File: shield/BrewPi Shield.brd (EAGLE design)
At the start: 53.6 x 59.7 mm, 30 parts, among them J1 ARDUINO_R3_SHIELD_ICSP, Q1 2N3906, U1 SN74HC595N

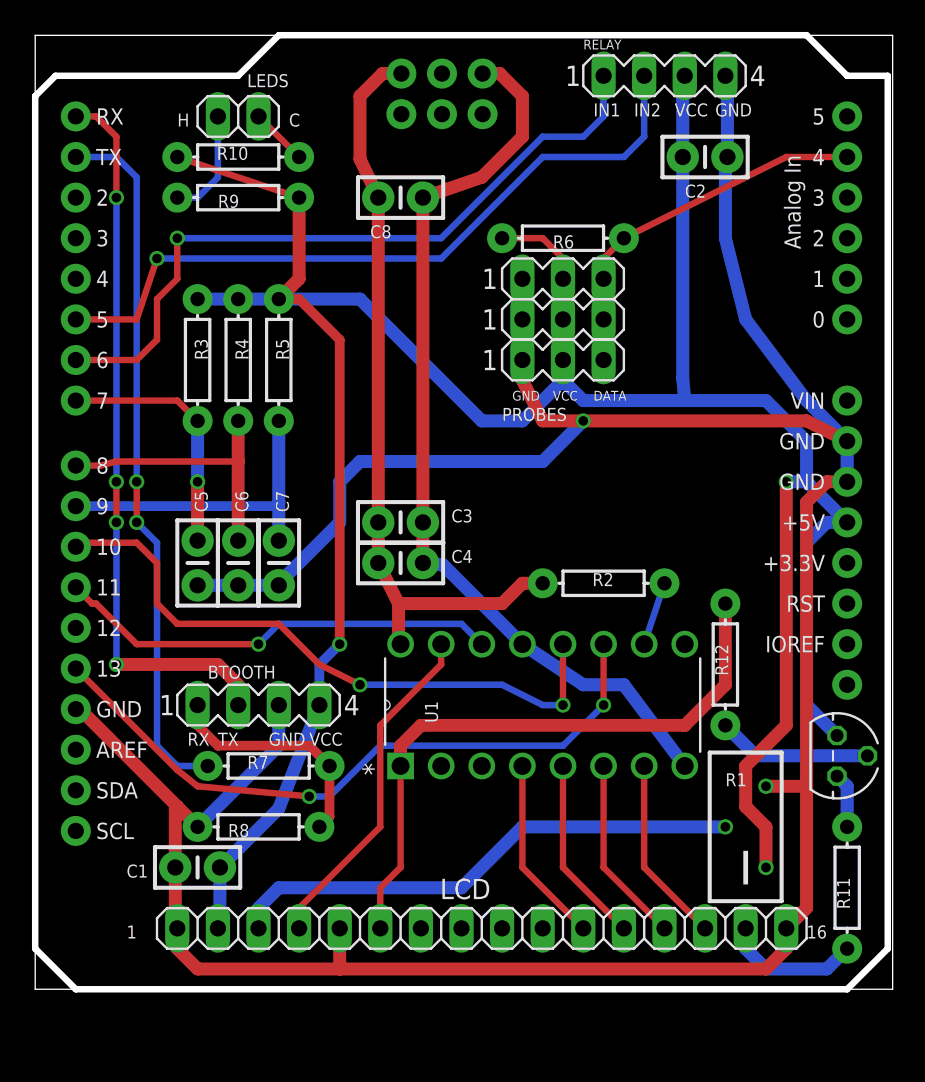
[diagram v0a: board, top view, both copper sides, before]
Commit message: Version 1.3 upload
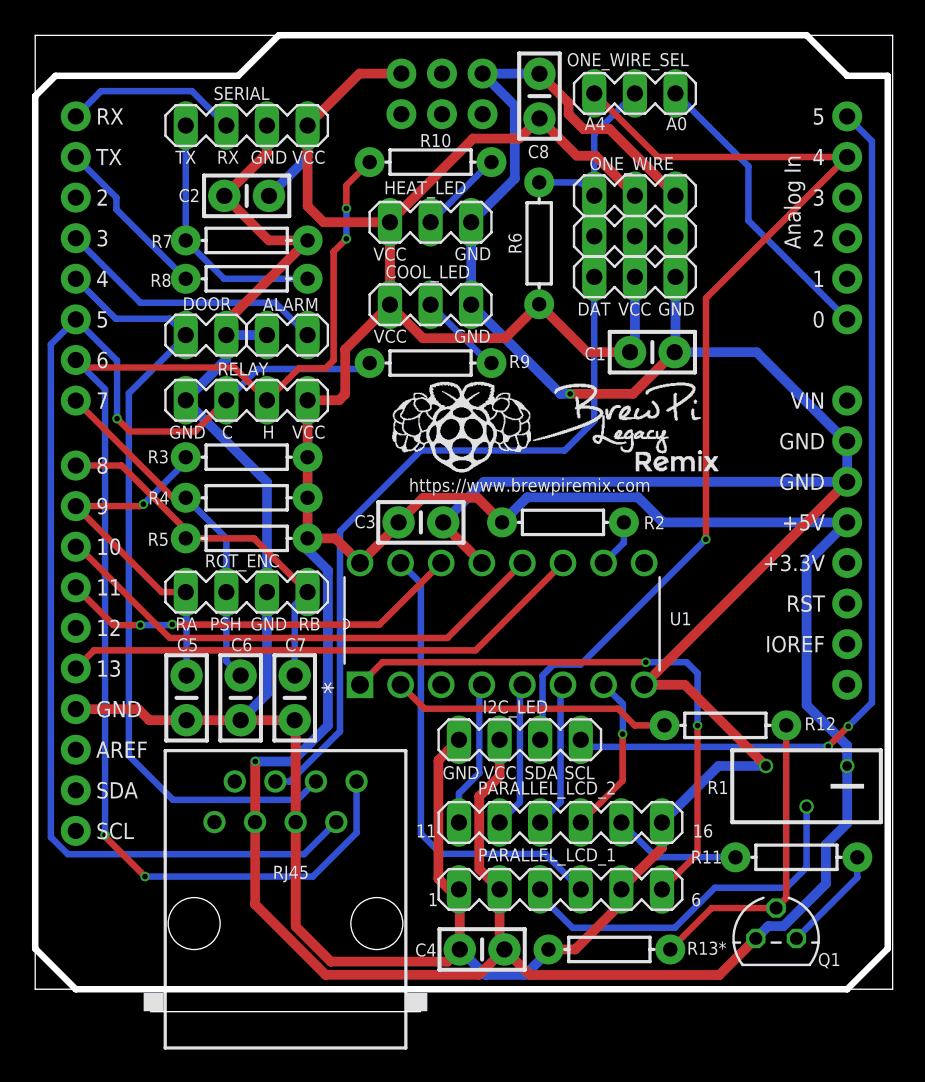
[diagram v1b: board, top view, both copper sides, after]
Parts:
- removed BTOOTH: (no value), con-lstb:MA04-1
- removed LCD: 16 pin, pinhead:1X16
- removed LEDS: (no value), pinhead:1X02
- added ALARM, DOOR: 2 pin, LBussy:HEADER02-1
- added COOL_LED, HEAT_LED, ONE_WIRE_SEL: 3 pin, LBussy:HEADER03-1
- added I2C_LED, ROT_ENC, SERIAL: 4 pin, LBussy:HEADER04-1
- added PARALLEL_LCD_1, PARALLEL_LCD_2: 6 pin, LBussy:HEADER06-1
- added R13*: 10kΩ, SparkFun-Passives:AXIAL-0.3
- added RJ45: RJ45-8X, con-tycoelectronics:RJ45-NO-SHIELD
- C1, C2, C3, C4: value .1UF -> 0.1μF
- C5, C6, C7: value (none) -> 0.1μF
- C8: value 1.0UF -> 1.0μF
- PROBE1, PROBE2, PROBE3: value (none) -> 3 pin; device con-lstb:MA03-1 -> LBussy:HEADER03-1
- R1, R3, R4, R5: value 10K -> 10kΩ
- R10, R9: value 220 -> 220Ω
- R11: value 470 Ohm -> 150Ω
- R12: value 10k Ohm -> 10kΩ
- R2: value 0-20K -> 20kΩ
- R6: value 4.7K -> 4.7kΩ
- R7: value 1K -> 2kΩ
- R8: value 2K -> 1kΩ
- RELAY: value (none) -> 4 pin; device con-lstb:MA04-1 -> LBussy:HEADER04-1
- moved C1 43.0 mm to (62.7, 58.9), turned to 0 degrees
- moved R8 34.3 mm to (37.4, 63.5), turned to 180 degrees
- moved RELAY 33.1 mm to (37.4, 55.9)
- moved R7 32.9 mm to (37.4, 65.9)
- moved C2 28.8 mm to (37.4, 68.7), turned to 180 degrees
- moved C4 24.7 mm to (52.1, 21.5), turned to 180 degrees
- moved R9 15.9 mm to (48.9, 58.2)
- moved Q1 12.0 mm to (70.5, 22.2), turned to 0 degrees
- moved R10 12.0 mm to (48.9, 70.8)
- moved R5 11.3 mm to (37.4, 47.3), turned to 0 degrees
- moved C8 10.8 mm to (55.7, 74.9), turned to 90 degrees
- moved R4 8.64 mm to (37.4, 49.8), turned to 0 degrees
- moved C7 8.50 mm to (40.4, 37.3)
- moved C5 8.47 mm to (33.6, 37.3)
- moved C6 8.44 mm to (37.0, 37.3)
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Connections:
- removed net 5V: BTOOTH.4, C1.1, C2.1, J1.5V, LCD.2, PROBE1.2, PROBE2.2, PROBE3.2, Q1.3, R1.1, R10.P$2, R3.P$2, R4.P$2, R5.P$2, R6.P$1, R9.P$2, RELAY.3
- removed net A5V: C3.1, C4.1, C8.1, J1.5V_ICSP, R2.P$2, U1.16
- removed net AGND: C3.2, C4.2, C8.2, J1.GND_ICSP, U1.13, U1.8
- removed net D5: J1.D5, RELAY.2
- removed net D6: J1.D6, RELAY.1
- removed net D7: C5.1, J1.D7, R3.P$1
- removed net IO8: C6.1, J1.D8, R4.P$1
- removed net IO9: C7.1, J1.D9, R5.P$1
- removed net N$12: LEDS.1, R9.P$1
- removed net N$13: LEDS.2, R10.P$1
- new net 1WIRE: ONE_WIRE_SEL.2, PROBE1.3, PROBE2.3, PROBE3.3, R6.P$2, RJ45.4
- new net A0: J1.A0, ONE_WIRE_SEL.3
- new net A4: I2C_LED.3, J1.A4, ONE_WIRE_SEL.1
- new net A5: I2C_LED.4, J1.A5
- new net ALARM: ALARM.1, J1.D3
- new net COOL: J1.D5, R9.P$1, RELAY.2, RJ45.7
- new net DOOR: DOOR.1, J1.D4, RJ45.6
- new net HEAT: J1.D6, R10.P$2, RELAY.3, RJ45.8
- new net N$8: HEAT_LED.2, R10.P$1
- new net PSHB: C6.1, J1.D7, R4.P$1, ROT_ENC.2
- new net QC: R12.P$1, U1.2
- new net ROTA: C5.1, J1.D9, R3.P$1, ROT_ENC.1
- new net ROTB: C7.1, J1.D8, R5.P$1, ROT_ENC.4
- new net VCC: C1.1, C2.1, C3.1, C4.1, C8.1, COOL_LED.1, HEAT_LED.1, I2C_LED.2, J1.5V, J1.5V_ICSP, PARALLEL_LCD_1.2, PROBE1.2, PROBE2.2, PROBE3.2, Q1.3, R1.1, R2.P$2, R3.P$2, R4.P$2, R5.P$2, R6.P$1, RELAY.4, RJ45.3, SERIAL.4, U1.16
- net GND: now also ALARM.2, C3.2, C4.2, C8.2, COOL_LED.3, DOOR.2, HEAT_LED.3, I2C_LED.1, J1.GND_ICSP, PARALLEL_LCD_1.1, PARALLEL_LCD_1.5, PARALLEL_LCD_2.6, R13*.P$1, R7.P$1, RELAY.1, RJ45.5, ROT_ENC.3, SERIAL.3, U1.13, U1.8; no longer BTOOTH.3, LCD.1, LCD.16, LCD.5, R8.P$1, RELAY.4
- net N$2: now also R13*.P$2
- net N$3: now also R7.P$2, R8.P$1, SERIAL.1; no longer BTOOTH.1, R7.P$1, R8.P$2
- net N$4: now also COOL_LED.2, R9.P$2; no longer J1.A4, PROBE1.3, PROBE2.3, PROBE3.3, R6.P$2
- net N$5: now also PARALLEL_LCD_2.5; no longer LCD.15
- net N$6: now also PARALLEL_LCD_1.3; no longer LCD.3
- net QA: now also PARALLEL_LCD_1.4; no longer LCD.4
- net QB: now also PARALLEL_LCD_1.6; no longer LCD.6, R12.P$1
- net QE: now also PARALLEL_LCD_2.1; no longer LCD.11
- net QF: now also PARALLEL_LCD_2.2; no longer LCD.12
- net QG: now also PARALLEL_LCD_2.3; no longer LCD.13
- net QH: now also PARALLEL_LCD_2.4; no longer LCD.14
- net RX: now also SERIAL.2; no longer BTOOTH.2
- net TX: now also R8.P$2; no longer R7.P$2
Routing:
- net VCC: track 0.00 -> 239.9 mm, vias 0 -> 1
- net 5V: track 184.4 -> 0.00 mm, vias 2 -> 0
- net HEAT: track 0.00 -> 83.2 mm, vias 0 -> 4
- net COOL: track 0.00 -> 77.4 mm, vias 0 -> 1
- net GND: track 198.1 -> 261.7 mm
- net A4: track 0.00 -> 62.9 mm, vias 0 -> 1
- net 1WIRE: track 0.00 -> 62.0 mm
- net AGND: track 57.7 -> 0.00 mm
- net A5: track 0.00 -> 56.9 mm, vias 0 -> 2
- net DOOR: track 0.00 -> 49.5 mm
- net A5V: track 47.6 -> 0.00 mm
- net D5: track 45.3 -> 0.00 mm, vias 1 -> 0
- net D6: track 44.8 -> 0.00 mm, vias 1 -> 0
- net RX: track 45.5 -> 11.0 mm, vias 4 -> 0
- net TX: track 44.1 -> 10.5 mm, vias 2 -> 0
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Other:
- board text added: "11"
- board text added: "2"
- board text added: "3"
- board text added: "4"
- board text added: "5"
- board text added: "5 - GND 6 - DOOR 7 - COOL 8 - HEAT"
- board text added: "6"
- board text added: "7"
- board text added: "8"
- board text added: "A0"
- board text added: "A4"
- board text added: "BrewPi Remix I2C/RevC Shield @CadiBrewer v1.3 Inspired by @LBussy Based on a design by @day_trippr"
- board text added: "DAT"
- board text added: "ONE_WIRE"
- board text added: "PSH"
- board text added: "Q1"
- board text added: "RA"
- board text added: "RB"
- board text added: "RJ45 Pinout: 1 - 2 - 3 - VCC 4 - DATA"
- board text added: "SCL"
- board text added: "SDA"
- board text added: "https://www.brewpiremix.com"
- board text removed: "Based on a design by day_trippr on Homebrewtalk"
- board text removed: "BrewPi Shield v1.2"
- board text removed: "DATA"
- board text removed: "IN1"
- board text removed: "IN2"
- board text removed: "PROBES"
- board text removed: "by cadibrewer"
